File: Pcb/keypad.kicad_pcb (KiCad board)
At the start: 2 copper layers, 75 x 75 mm, 5 parts, among them SW1 SW_Push, SW2 SW_Push, SW3 SW_Push, SW4 SW_Push, U1 MOUDLE-SEEEDUINO-XIAO

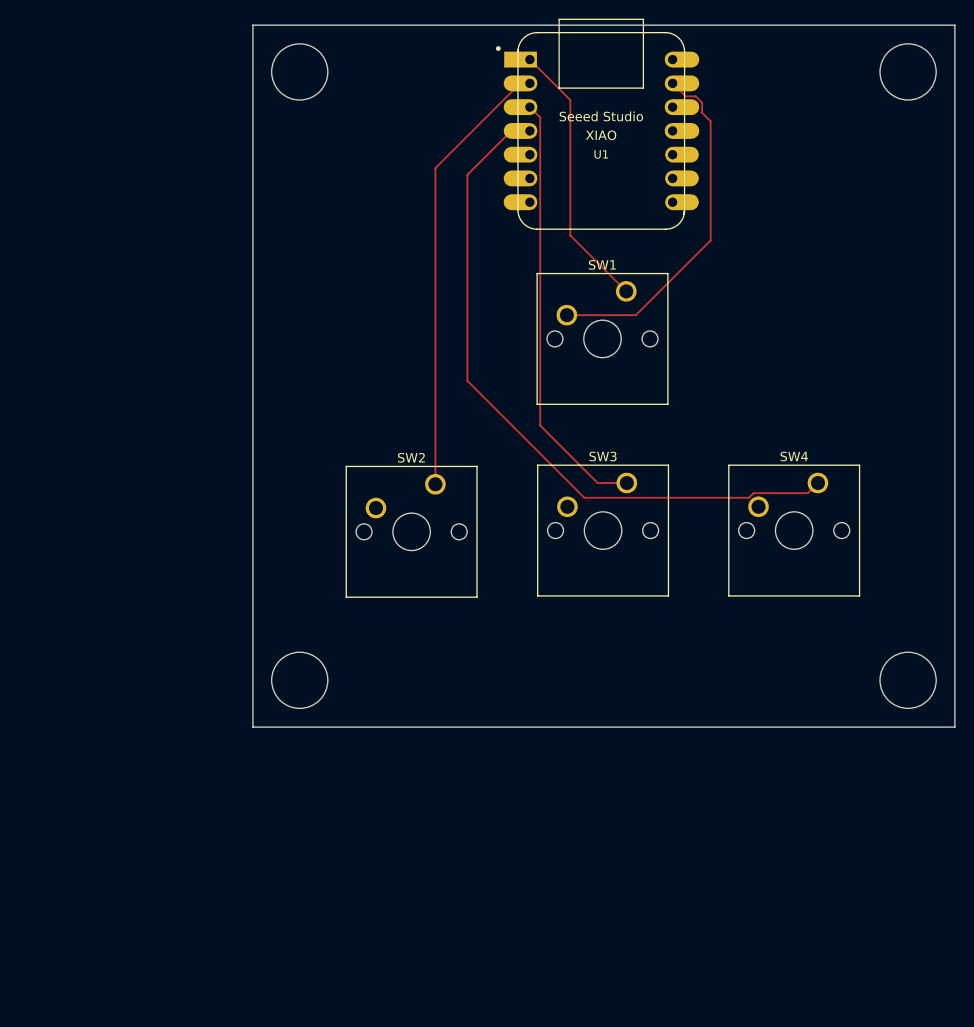
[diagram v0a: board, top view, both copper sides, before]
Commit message: pcb design
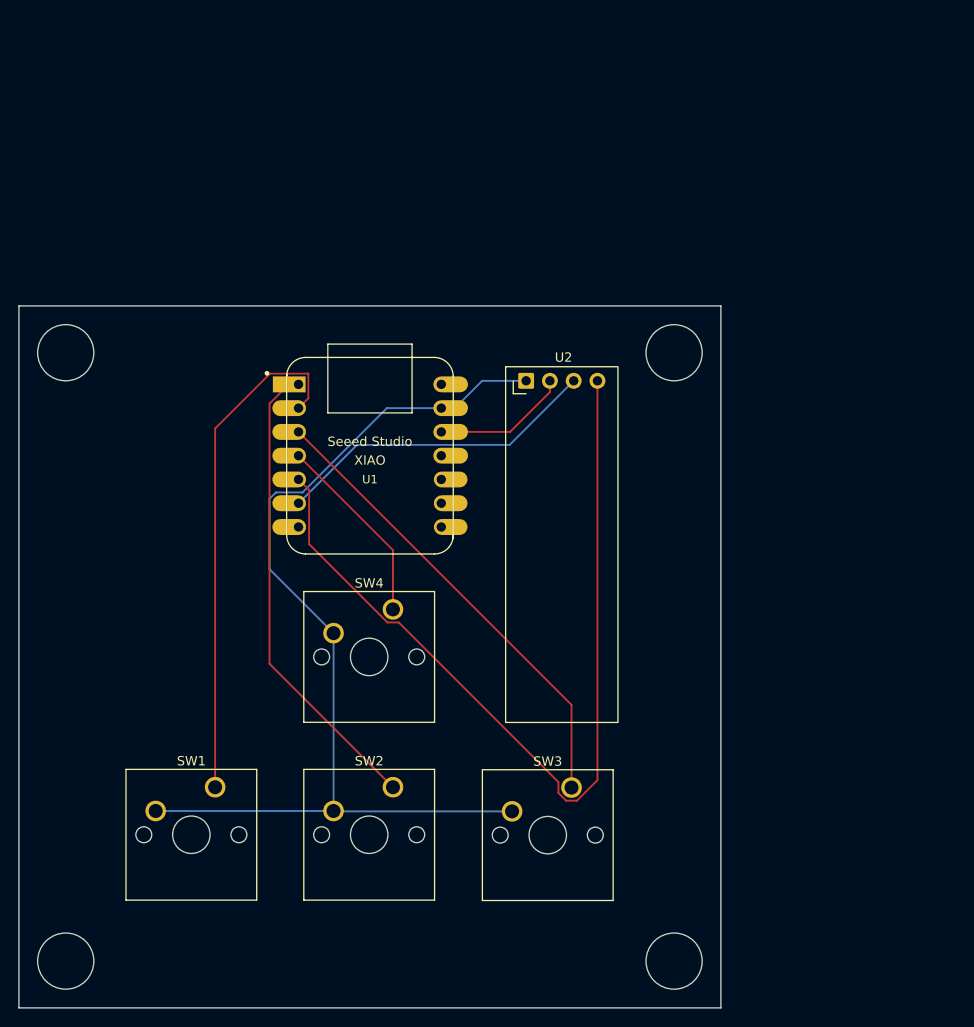
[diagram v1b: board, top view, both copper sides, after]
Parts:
- added U2: ER_OLEDM0.91_1x-I2C, Display:ER_OLEDM0.91_1x-I2C, F.Cu at (139.2, 58.0)
- moved SW1 68.8 mm to (106.0, 101.4)
- moved SW4 47.4 mm to (125.0, 82.4)
- moved U1 42.6 mm to (122.5, 66.0)
- moved SW3 33.1 mm to (144.0, 101.5)
- moved SW2 32.7 mm to (125.0, 101.4)
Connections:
- SW1 pad 1: Net-(U1-PA02_A0_D0) -> Net-(U1-PA4_A1_D1)
- SW2 pad 1: Net-(U1-PA4_A1_D1) -> Net-(U1-PA02_A0_D0)
- U1 pad 12: unconnected-(U1-3V3-Pad12) -> Net-(U1-3V3)
- U1 pad 5: unconnected-(U1-PA8_A4_D4_SDA-Pad5) -> Net-(U1-PA8_A4_D4_SDA)
- U1 pad 6: unconnected-(U1-PA9_A5_D5_SCL-Pad6) -> Net-(U1-PA9_A5_D5_SCL)
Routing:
- net Net-(U1-PA8_A4_D4_SDA): track 0.00 -> 93.8 mm
- net GND: track 37.8 -> 106.9 mm
- net Net-(U1-PA11_A3_D3): track 73.9 -> 20.6 mm
- net Net-(U1-PA9_A5_D5_SCL): track 0.00 -> 34.8 mm
- net Net-(U1-PA02_A0_D0): track 29.0 -> 50.4 mm
- net Net-(U1-3V3): track 0.00 -> 14.6 mm
- net Net-(U1-PA4_A1_D1): track 47.6 -> 54.8 mm
- net Net-(U1-PA10_A2_D2): track 46.3 -> 50.1 mm
